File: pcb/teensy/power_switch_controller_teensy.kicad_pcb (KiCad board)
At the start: 2 copper layers, 63.5 x 40.6 mm, 15 parts, among them P1 HEADER_02X08_SMD, SW1 SPST_SLIDE_AS, U1 TLE7230R

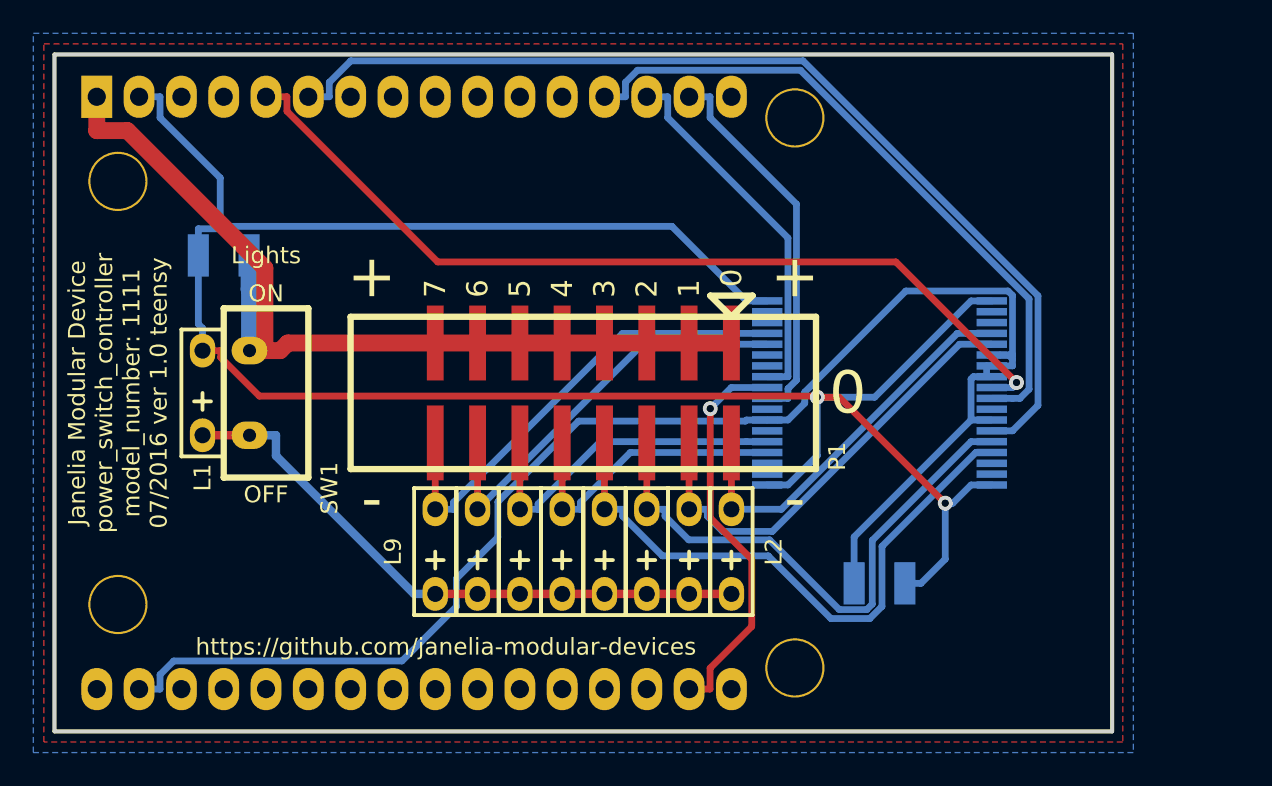
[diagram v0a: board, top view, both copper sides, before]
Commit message: Finished pcb v1.1.
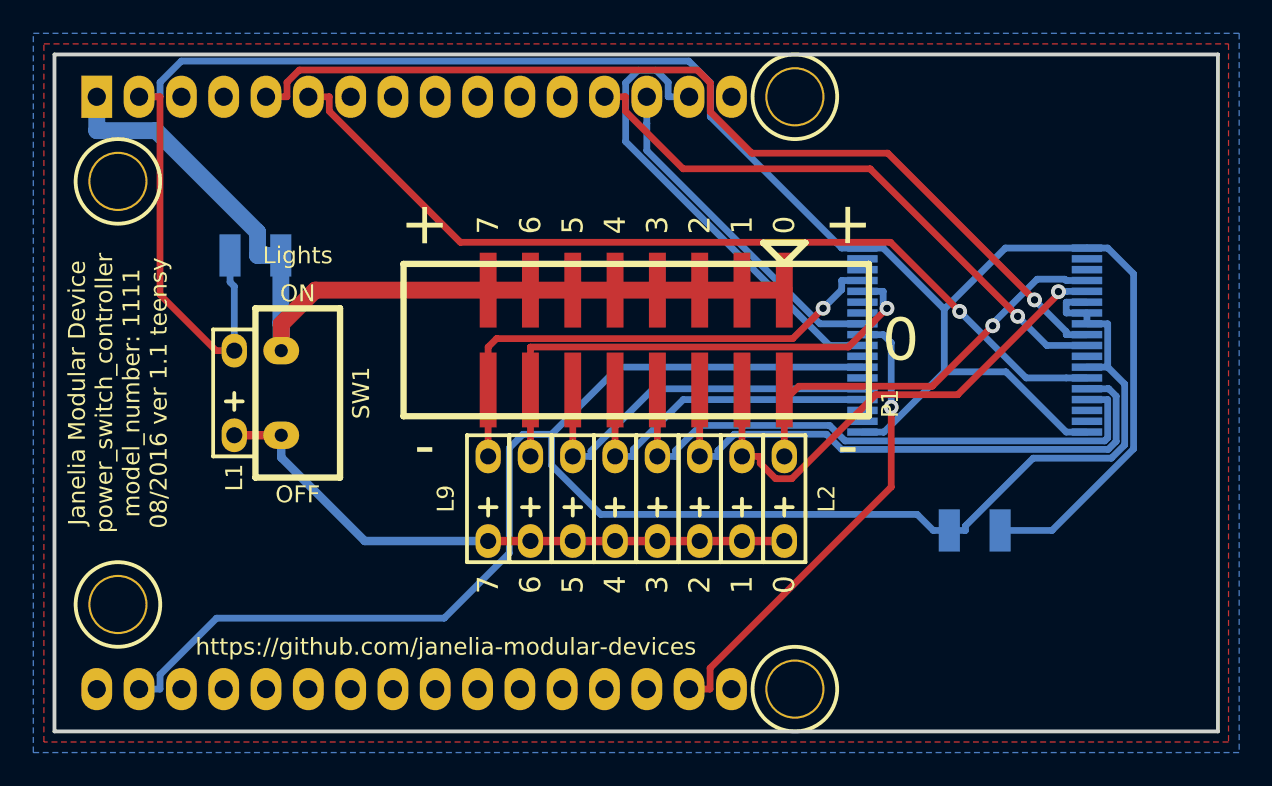
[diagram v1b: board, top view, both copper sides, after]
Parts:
- MDT1: footprint power_switch_controller_teensy:MODULAR_DEVICE_TEENSY -> power_switch_controller_teensy:MODULAR_DEVICE_TEENSY_MALE
- moved C2 6.54 mm to (128.9, 108.0)
- moved U1 6.54 mm to (128.9, 96.5)
- moved L7 4.49 mm to (104.8, 106.0)
- moved L2 4.49 mm to (117.5, 106.0)
- moved L3 4.49 mm to (114.9, 106.0)
- moved L4 4.49 mm to (112.4, 106.0)
- moved L5 4.49 mm to (109.9, 106.0)
- moved L6 4.49 mm to (107.3, 106.0)
- moved L8 4.49 mm to (102.2, 106.0)
- moved L9 4.49 mm to (99.7, 106.0)
- moved P1 4.49 mm to (108.6, 96.5)
- moved C1 1.91 mm to (85.7, 91.4)
- moved L1 1.91 mm to (84.5, 99.7)
- moved SW1 1.91 mm to (88.3, 99.7)
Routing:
- net VEE: track 91.1 -> 109.8 mm
- net /PWM: track 61.0 -> 54.2 mm, vias 0 -> 1
- net /OUT6: track 25.5 -> 31.3 mm, vias 0 -> 1
- net /MISO: track 23.0 -> 28.1 mm
- net /CS: track 40.2 -> 35.7 mm, vias 0 -> 1
- net /SCK: track 24.1 -> 28.5 mm
- net /RESET: track 54.3 -> 58.2 mm
- net GND: track 132.4 -> 136.2 mm, vias 2 -> 0
- net /OUT1: track 27.6 -> 30.2 mm, vias 0 -> 1
- net /OUT5: track 20.7 -> 23.2 mm
- net /OUT4: track 18.0 -> 20.5 mm
- net /OUT7: track 28.5 -> 31.0 mm, vias 0 -> 1
- net /MOSI: track 22.3 -> 20.5 mm
- net /OUT0: track 24.0 -> 25.3 mm, vias 0 -> 1
- net /OUT2: track 33.8 -> 35.0 mm
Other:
- board size 63.5 x 40.6 mm -> 69.8 x 40.6 mm
- board text added: "Janelia Modular Device power_switch_controller model_number: 1111 08/2016 ver 1.1 teensy"
- board text removed: "Janelia Modular Device power_switch_controller model_number: 1111 07/2016 ver 1.0 teensy"
